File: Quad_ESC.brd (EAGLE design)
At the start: 96.5 x 40.1 mm, 28 parts, among them Y1 ECS-80-S-4X

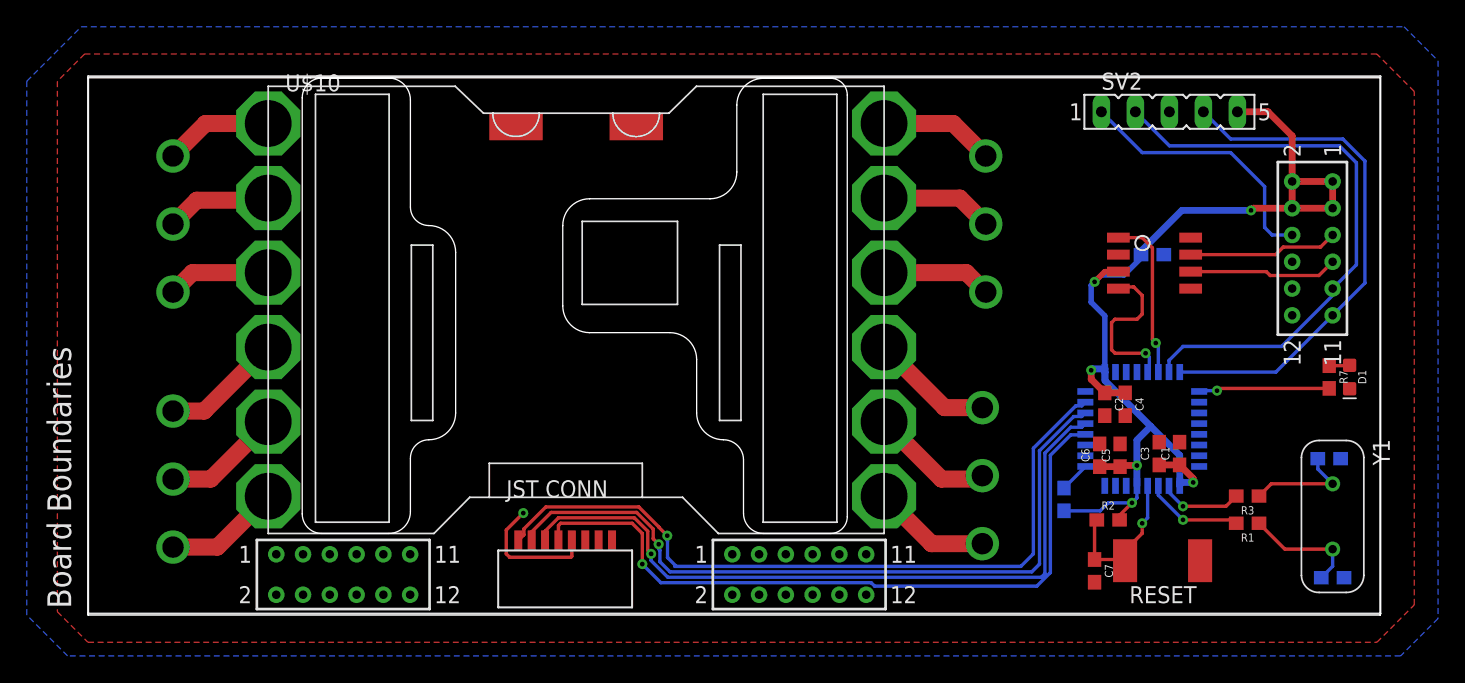
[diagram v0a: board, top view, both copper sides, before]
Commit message: Board Update (again)
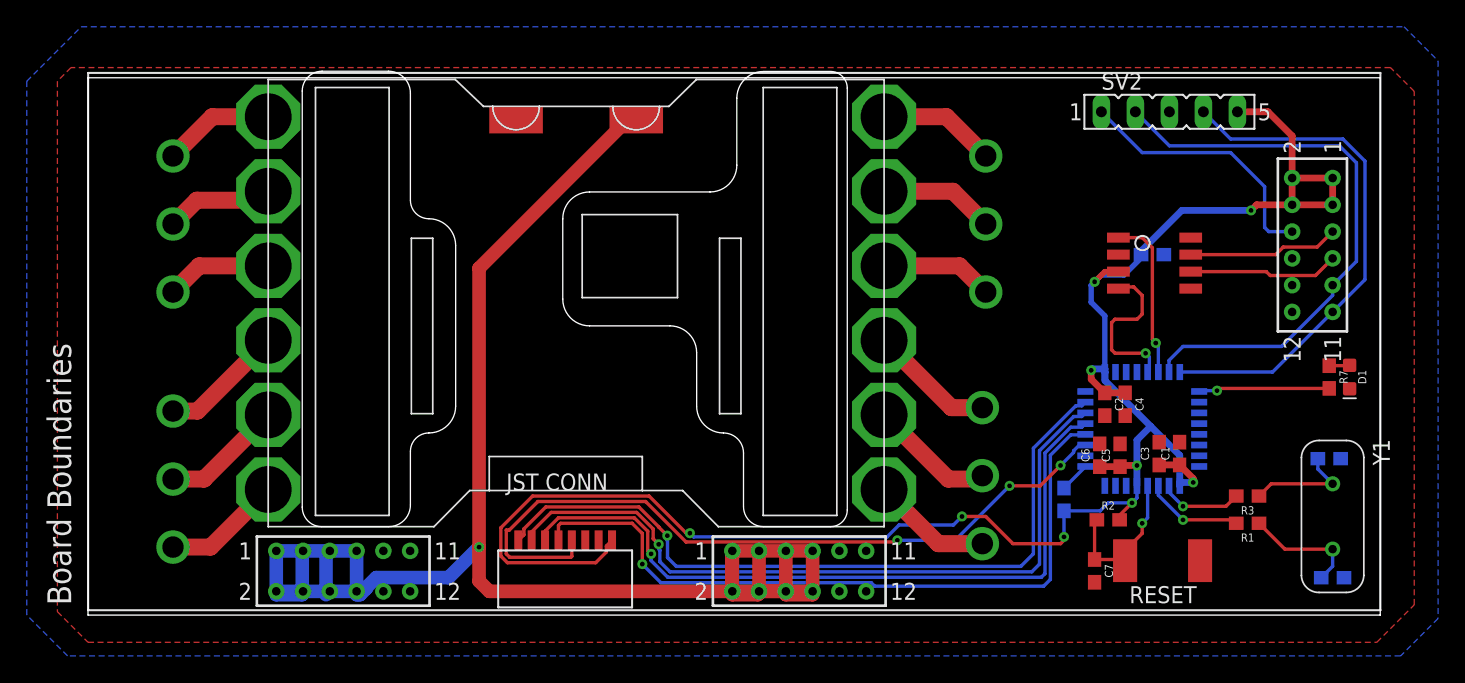
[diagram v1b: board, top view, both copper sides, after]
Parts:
- moved U$10 0.51 mm to (13.5, 6.60)
- moved U$3 0.25 mm to (19.1, 3.28)
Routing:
- net +12V: track 0.00 -> 129.6 mm, vias 0 -> 1
- net +3V3: track 81.4 -> 140.9 mm, vias 6 -> 9
- net TLM: track 9.79 -> 56.5 mm, vias 1 -> 3
- net ESC1_Y: track 7.34 -> 8.22 mm
- net ESC4_Y: track 8.61 -> 9.43 mm
